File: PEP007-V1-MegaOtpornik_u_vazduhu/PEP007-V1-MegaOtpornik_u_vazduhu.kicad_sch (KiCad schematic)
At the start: 8 parts, among them J2 Klema

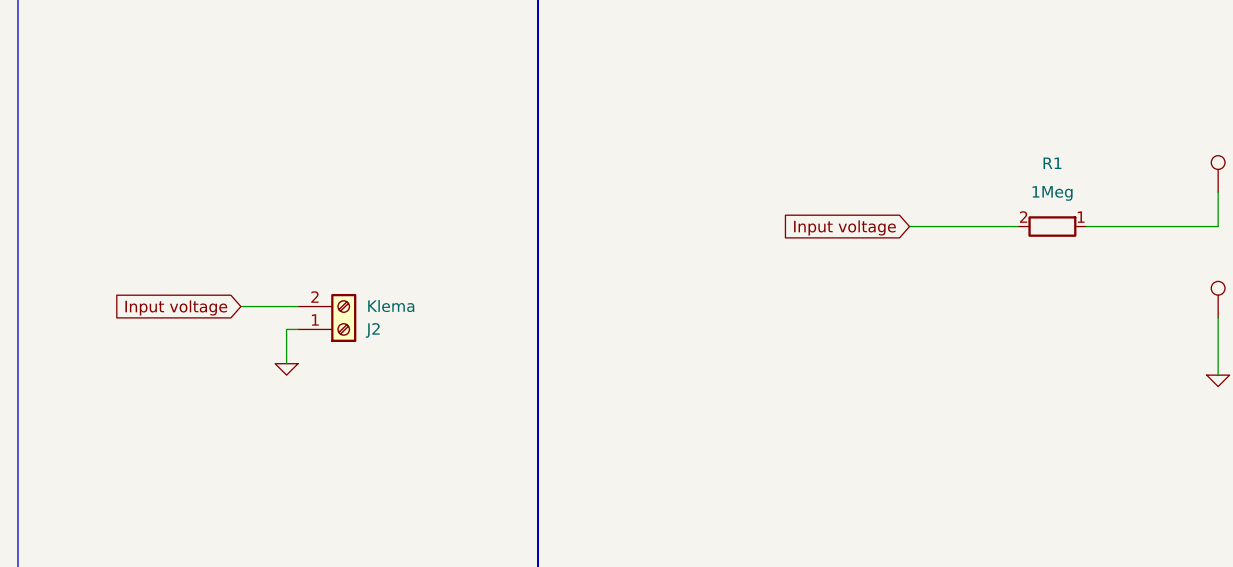
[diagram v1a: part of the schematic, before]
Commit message: Update 1,2,3,4,5,7, lib.
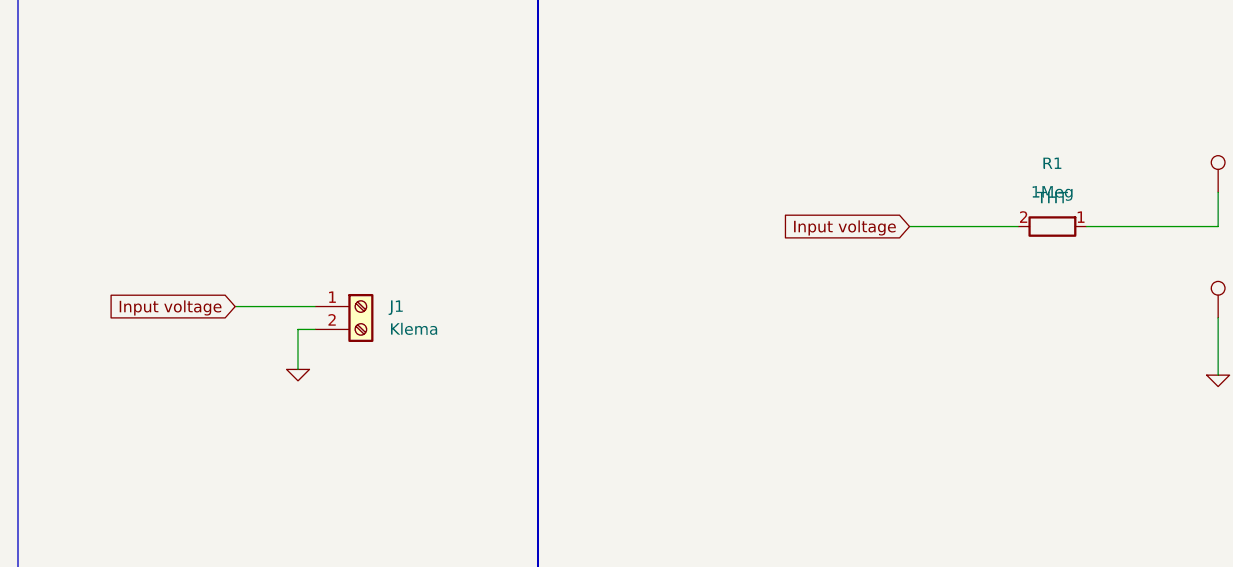
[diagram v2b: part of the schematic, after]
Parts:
- removed J2: Klema, PEP_library:TerminalBlock_Phoenix_MKDS-1,5-2-5.08_1x02_P5.08mm_Horizontal, symbol PEP_library:Klema
- added J1: Klema, PEP_library:TerminalBlock_Phoenix_MKDS-1,5-2-5.08_1x02_P5.08mm_Horizontal, symbol PEP_library:Klema
- R1: Size (none) -> THT
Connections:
- net 0: now also J1.2 (Pin_2)
- net Input voltage: now also J1.1 (Pin_1)
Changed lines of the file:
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@@
 (kicad_sch
-	(version 20231120)
+	(version 20250114)
 	(generator "eeschema")
-	(generator_version "8.0")
+	(generator_version "9.0")
 	(paper "A5")
 	(title_block
@@
 		(rev "v1")
 	)
-	(wire
-		(pts
-			(xy 145.415 55.88) (xy 130.81 55.88)
-		)
-		(stroke
-			(width 0)
-			(type default)
-		)
-	)
-	(wire
-		(pts
-			(xy 41.91 67.31) (xy 41.91 71.12)
-		)
-		(stroke
-			(width 0)
-			(type default)
-		)
-	)
-	(wire
-		(pts
-			(xy 111.125 55.88) (xy 123.19 55.88)
-		)
-		(stroke
-			(width 0)
-			(type default)
-		)
-	)
-	(wire
-		(pts
-			(xy 36.83 64.77) (xy 43.18 64.77)
-		)
-		(stroke
-			(width 0)
-			(type default)
-		)
-	)
-	(wire
-		(pts
-			(xy 145.415 66.04) (xy 145.415 72.39)
-		)
-		(stroke
-			(width 0)
-			(type default)
-		)
-	)
-	(wire
-		(pts
-			(xy 41.91 67.31) (xy 43.18 67.31)
-		)
-		(stroke
-			(width 0)
-			(type default)
-		)
-	)
-	(wire
-		(pts
-			(xy 145.415 52.07) (xy 145.415 55.88)
-		)
-		(stroke
-			(width 0)
-			(type default)
-		)
-	)
 	(rectangle
 		(start 12.065 12.065)
@@
 		)
 	)
+	(wire
+		(pts
+			(xy 145.415 55.88) (xy 130.81 55.88)
+		)
+		(stroke
+			(width 0)
+			(type default)
+		)
+	)
+	(wire
+		(pts
+			(xy 43.18 67.31) (xy 45.085 67.31)
+		)
+		(stroke
+			(width 0)
+			(type default)
+		)
+	)
+	(wire
+		(pts
+			(xy 111.125 55.88) (xy 123.19 55.88)
+		)
+		(stroke
+			(width 0)
+			(type default)
+		)
+	)
+	(wire
+		(pts
+			(xy 36.195 64.77) (xy 45.085 64.77)
+		)
+		(stroke
+			(width 0)
+			(type default)
+		)
+	)
+	(wire
+		(pts
+			(xy 145.415 66.04) (xy 145.415 72.39)
+		)
+		(stroke
+			(width 0)
+			(type default)
+		)
+	)
+	(wire
+		(pts
+			(xy 43.18 67.31) (xy 43.18 71.755)
+		)
+		(stroke
+			(width 0)
+			(type default)
+		)
+	)
+	(wire
+		(pts
+			(xy 145.415 52.07) (xy 145.415 55.88)
+		)
+		(stroke
+			(width 0)
+			(type default)
+		)
+	)
 	(global_label "Input voltage"
 		(shape input)
-		(at 36.83 64.77 180)
+		(at 36.195 64.77 180)
 		(fields_autoplaced yes)
 		(effects
@@
 		)
 		(property "Intersheetrefs" "${INTERSHEET_REFS}"
-			(at 21.2056 64.77 0)
+			(at 20.5706 64.77 0)
 			(effects
 				(font
@@
 	(symbol
 		(lib_id "Simulation_SPICE:0")
-		(at 41.91 71.12 0)
+		(at 43.18 71.755 0)
 		(mirror y)
 		(unit 1)
@@
 		(dnp no)
 		(fields_autoplaced yes)
-		(property "Reference" "#GND05"
-			(at 41.91 73.66 0)
+		(property "Reference" "#GND0102"
+			(at 43.18 74.295 0)
 			(effects
 				(font
@@
 		)
 		(property "Value" "0"
-			(at 41.91 68.58 0)
+			(at 43.18 69.215 0)
 			(effects
 				(font
@@
 		)
 		(property "Footprint" ""
-			(at 41.91 71.12 0)
-			(effects
-				(font
-					(size 1.27 1.27)
-				)
-				(hide yes)
-			)
-		)
-		(property "Datasheet" "~"
-			(at 41.91 71.12 0)
-			(effects
-				(font
-					(size 1.27 1.27)
-				)
-				(hide yes)
-			)
-		)
-		(property "Description" ""
-			(at 41.91 71.12 0)
+			(at 43.18 71.755 0)
+			(effects
+				(font
+					(size 1.27 1.27)
+				)
+				(hide yes)
+			)
+		)
+		(property "Datasheet" "https://ngspice.sourceforge.io/docs/ngspice-html-manual/manual.xhtml#subsec_Circuit_elements__device"
+			(at 43.18 71.755 0)
+			(effects
+				(font
+					(size 1.27 1.27)
+				)
+				(hide yes)
+			)
+		)
+		(property "Description" "0V reference potential for simulation"
+			(at 43.18 71.755 0)
 			(effects
 				(font
@@
 			(project "006_RC_vremenska_konstanta"
 				(path "/4bec5ddf-adbf-41fb-a069-c7630bb0044a"
-					(reference "#GND05")
+					(reference "#GND0102")
 					(unit 1)
 				)
@@
 			)
 		)
-		(property "Description" ""
+		(property "Description" "Mounting Hole without connection"
 			(at 30.48 127 0)
 			(effects
@@
 				(path "/4bec5ddf-adbf-41fb-a069-c7630bb0044a"
 					(reference "H3")
-					(unit 1)
-				)
-			)
-		)
-	)
-	(symbol
-		(lib_id "PEP_library:Klema")
-		(at 48.26 67.31 0)
-		(mirror x)
-		(unit 1)
-		(exclude_from_sim no)
-		(in_bom yes)
-		(on_board yes)
-		(dnp no)
-		(fields_autoplaced yes)
-		(property "Reference" "J2"
-			(at 50.8 67.3101 0)
-			(effects
-				(font
-					(size 1.27 1.27)
-				)
-				(justify left)
-			)
-		)
-		(property "Value" "Klema"
-			(at 50.8 64.7701 0)
-			(effects
-				(font
-					(size 1.27 1.27)
-				)
-				(justify left)
-			)
-		)
-		(property "Footprint" "PEP_library:TerminalBlock_Phoenix_MKDS-1,5-2-5.08_1x02_P5.08mm_Horizontal"
-			(at 48.26 67.31 0)
-			(effects
-				(font
-					(size 1.27 1.27)
-				)
-				(hide yes)
-			)
-		)
-		(property "Datasheet" "~"
-			(at 48.26 67.31 0)
-			(effects
-				(font
-					(size 1.27 1.27)
-				)
-				(hide yes)
-			)
-		)
-		(property "Description" "Generic screw terminal, single row, 01x02, script generated (kicad-library-utils/schlib/autogen/connector/)"
-			(at 48.26 67.31 0)
-			(effects
-				(font
-					(size 1.27 1.27)
-				)
-				(hide yes)
-			)
-		)
-		(property "LCSC" "C474952"
-			(at 48.26 67.31 0)
-			(effects
-				(font
-					(size 1.27 1.27)
-				)
-				(hide yes)
-			)
-		)
-		(pin "1"
-		)
-		(pin "2"
-		)
-		(instances
-			(project ""
-				(path "/4bec5ddf-adbf-41fb-a069-c7630bb0044a"
-					(reference "J2")
 					(unit 1)
 				)
@@
 	)
 	(symbol
+		(lib_id "PEP_library:Klema")
+		(at 50.165 64.77 0)
+		(unit 1)
+		(exclude_from_sim no)
+		(in_bom yes)
+		(on_board yes)
+		(dnp no)
+		(fields_autoplaced yes)
+		(property "Reference" "J1"
+			(at 53.34 64.7699 0)
+			(effects
+				(font
+					(size 1.27 1.27)
+				)
+				(justify left)
+			)
+		)
+		(property "Value" "Klema"
+			(at 53.34 67.3099 0)
+			(effects
+				(font
+					(size 1.27 1.27)
+				)
+				(justify left)
+			)
+		)
+		(property "Footprint" "PEP_library:TerminalBlock_Phoenix_MKDS-1,5-2-5.08_1x02_P5.08mm_Horizontal"
+			(at 50.165 64.77 0)
+			(effects
+				(font
+					(size 1.27 1.27)
+				)
+				(hide yes)
+			)
+		)
+		(property "Datasheet" "~"
+			(at 50.165 64.77 0)
+			(effects
+				(font
+					(size 1.27 1.27)
+				)
+				(hide yes)
+			)
+		)
+		(property "Description" "Generic screw terminal, single row, 01x02, script generated (kicad-library-utils/schlib/autogen/connector/)"
+			(at 50.165 64.77 0)
+			(effects
+				(font
+					(size 1.27 1.27)
+				)
+				(hide yes)
+			)
+		)
+		(pin "1"
+		)
+		(pin "2"
+		)
+		(instances
+			(project ""
+				(path "/4bec5ddf-adbf-41fb-a069-c7630bb0044a"
+					(reference "J1")
+					(unit 1)
+				)
+			)
+		)
+	)
+	(symbol
 		(lib_id "Mechanical:MountingHole")
 		(at 49.53 119.38 0)
@@
 			)
 		)
-		(property "Description" ""
+		(property "Description" "Mounting Hole without connection"
 			(at 49.53 119.38 0)
 			(effects
@@
 		(dnp no)
 		(fields_autoplaced yes)
-		(property "Reference" "#GND01"
+		(property "Reference" "#GND0101"
 			(at 145.415 74.93 0)
 			(effects
@@
 			)
 		)
-		(property "Datasheet" "~"
+		(property "Datasheet" "https://ngspice.sourceforge.io/docs/ngspice-html-manual/manual.xhtml#subsec_Circuit_elements__device"
 			(at 145.415 72.39 0)
 			(effects
@@
 			)
 		)
-		(property "Description" ""
+		(property "Description" "0V reference potential for simulation"
 			(at 145.415 72.39 0)
 			(effects
@@
 			(project "PEP007-V1-MegaOtpornik_u_vazduhu"
 				(path "/4bec5ddf-adbf-41fb-a069-c7630bb0044a"
-					(reference "#GND01")
+					(reference "#GND0101")
 					(unit 1)
 				)
@@
 			)
 		)
-		(property "Description" ""
+		(property "Description" "Mounting Hole without connection"
 			(at 30.48 119.38 0)
 			(effects
@@
 			)
 		)
-		(property "Description" ""
+		(property "Description" "Mounting Hole without connection"
 			(at 49.53 127 0)
 			(effects
@@
 			)
 		)
-		(property "Size" ""
+		(property "Size" "THT"
 			(at 127 52.705 90)
 			(effects
@@
 		)
 	)
+	(embedded_fonts no)
 )
